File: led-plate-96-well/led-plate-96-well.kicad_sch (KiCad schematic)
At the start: 2 parts, among them U1 TLC5947RHB, U2 A000053

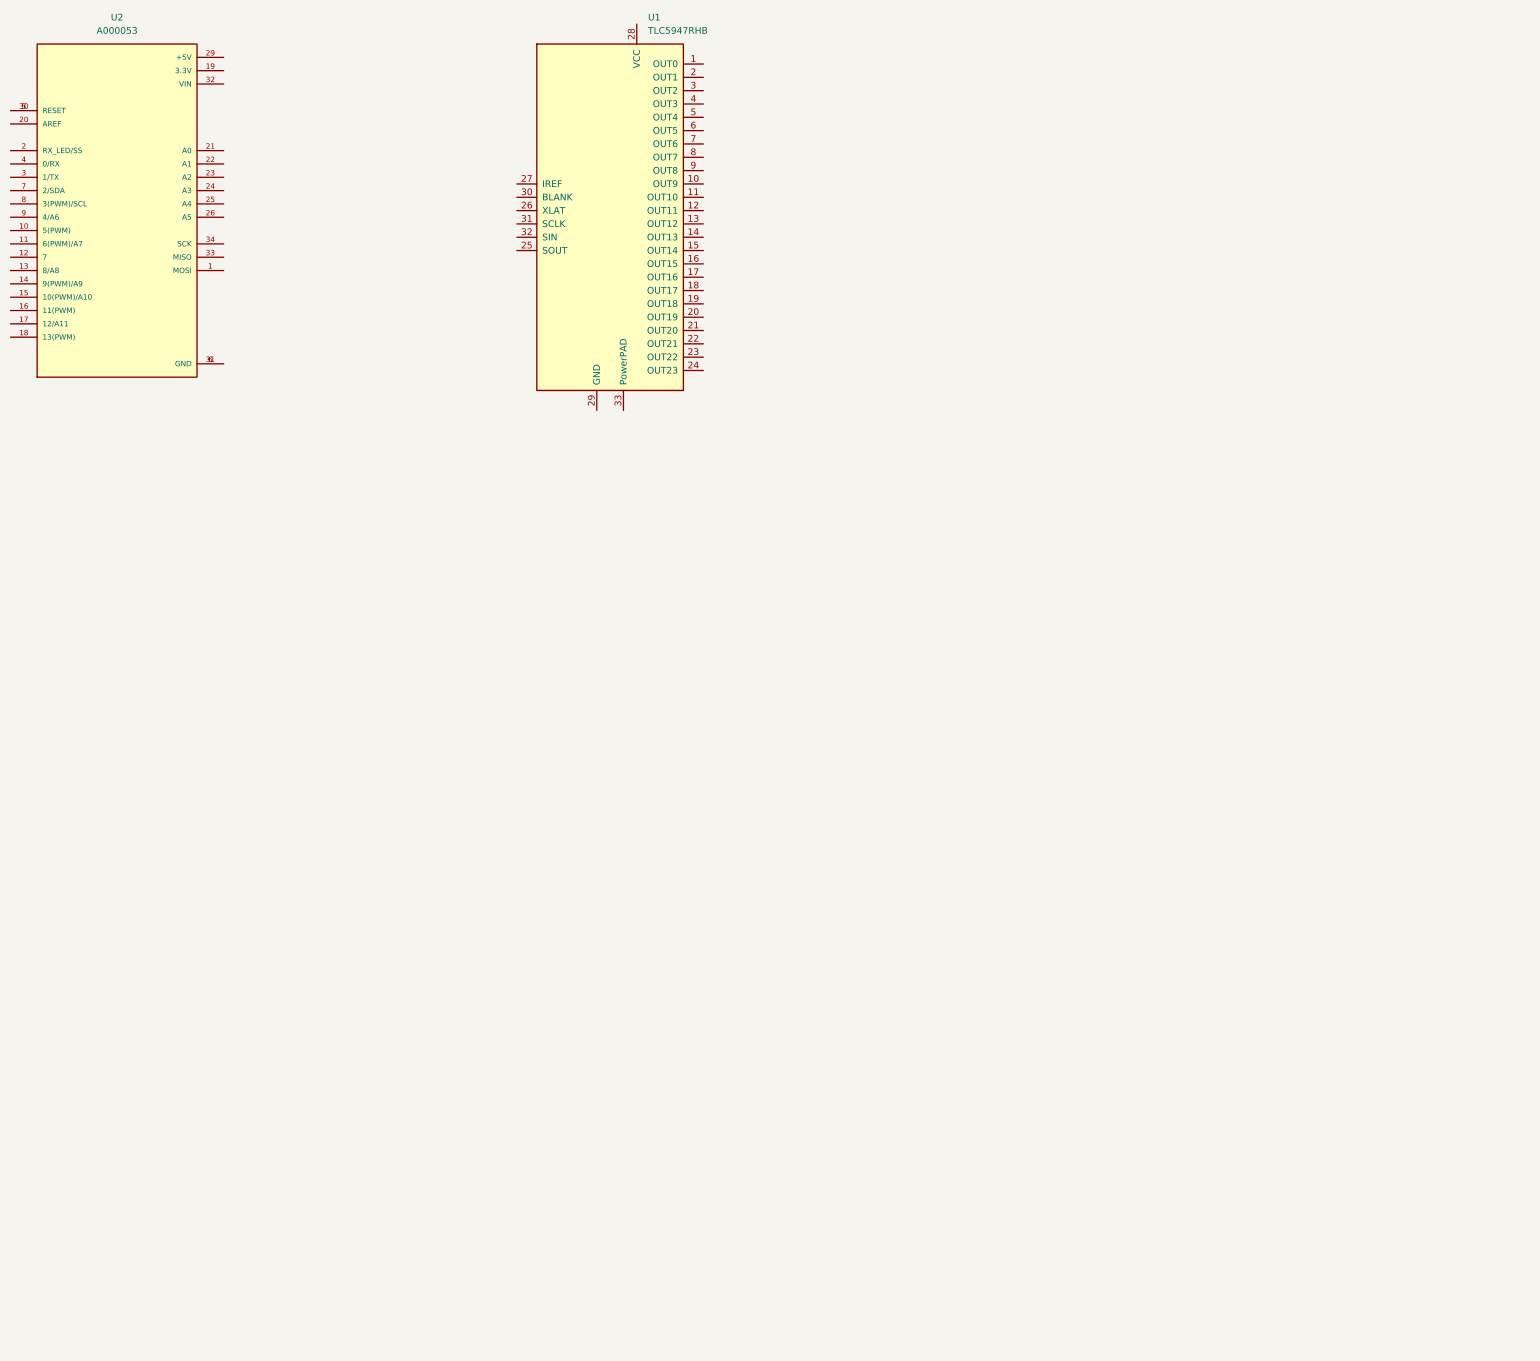
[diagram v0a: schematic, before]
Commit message: start main board
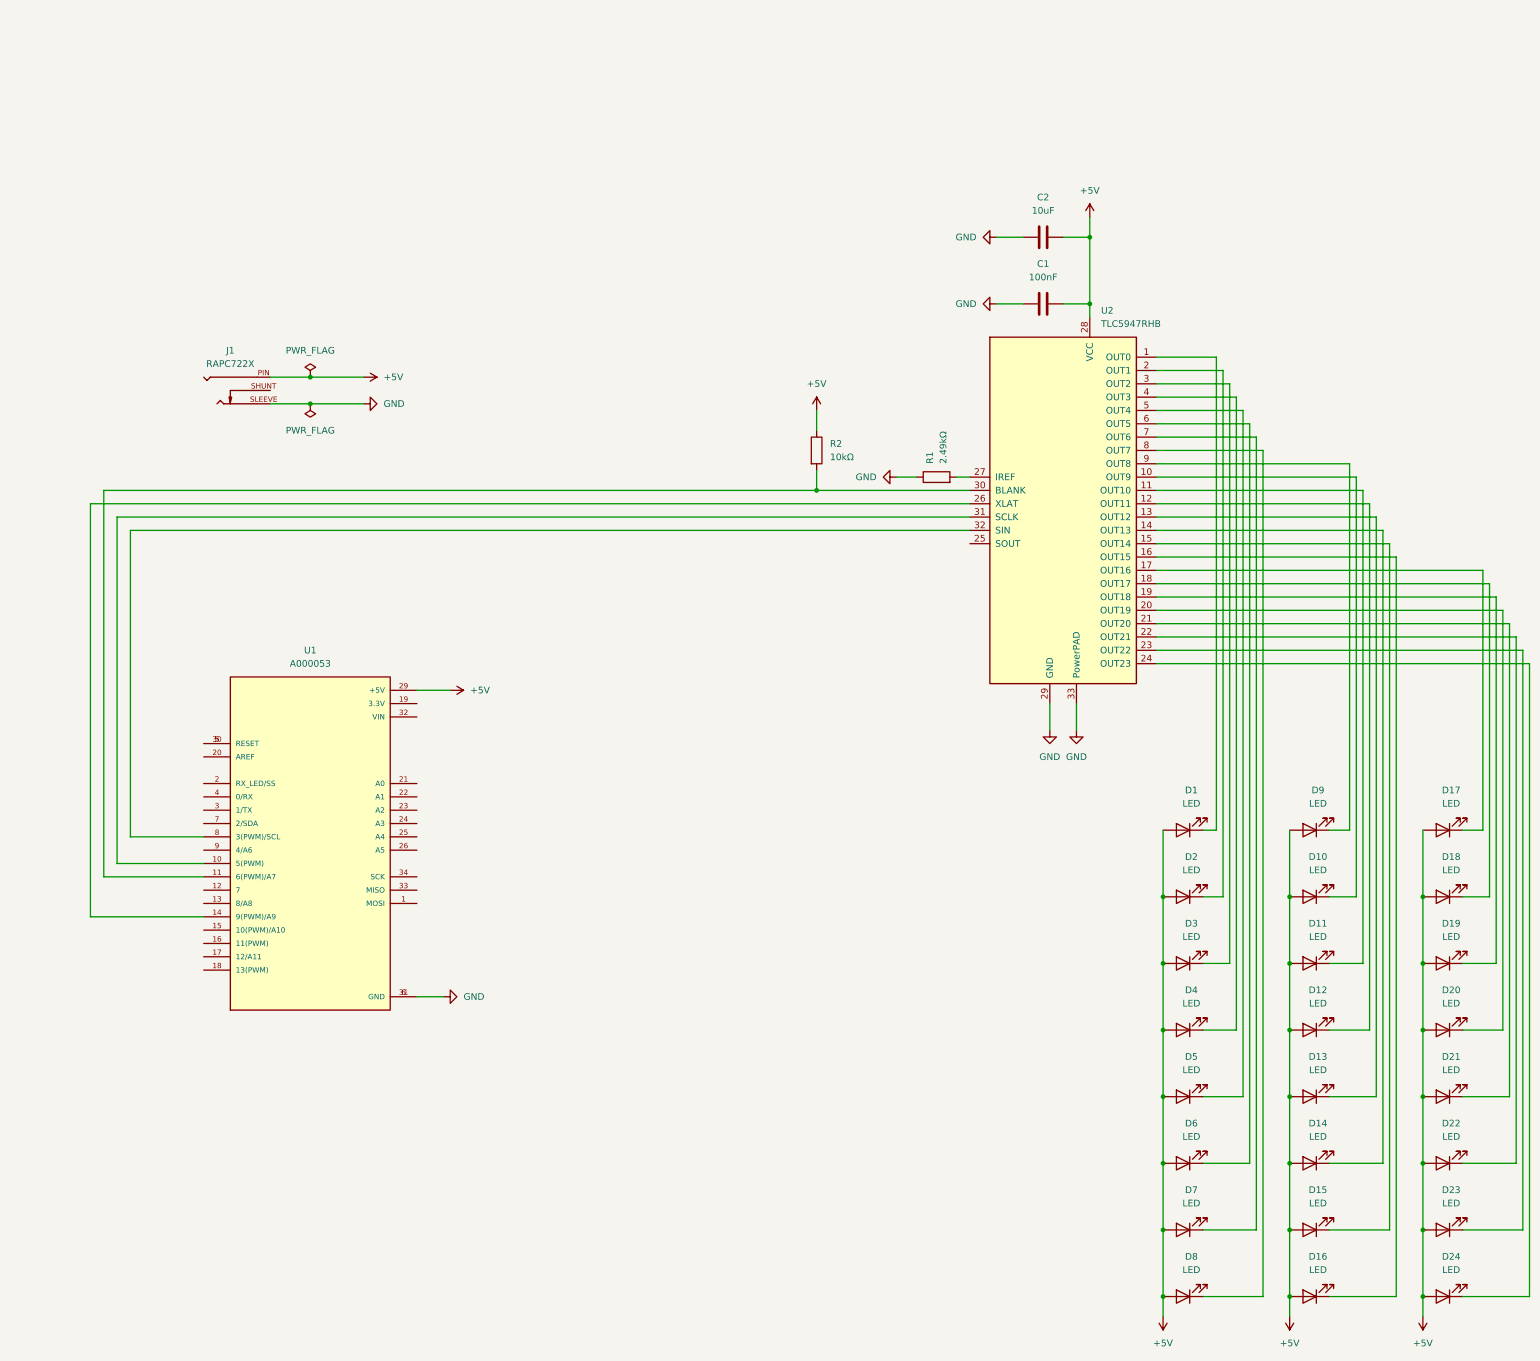
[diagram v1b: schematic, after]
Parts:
- added C1: 100nF, Capacitor_SMD:C_0603_1608Metric, symbol Device:C
- added C2: 10uF, Capacitor_SMD:C_0805_2012Metric, symbol Device:C
- added D1, D10, D11, D12, D13, D14, D15, D16, D17, D18, D19, D2, D20, D21, D22, D23, D24, D3, D4, D5, D6, D7, D8, D9: LED, SMD2835_WITH_STEP:LED_PLCC_2835, symbol Device:LED
- added J1: RAPC722X, RAPC722X:SWITCHCRAFT_RAPC722X, symbol RAPC722X:RAPC722X
- added R1: 2.49kΩ, Resistor_SMD:R_0402_1005Metric, symbol Device:R
- added R2: 10kΩ, Resistor_SMD:R_0603_1608Metric, symbol Device:R
- renumbered U2 to U1, U1 to U2
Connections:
- net at U1.10 (5(PWM)): now also U2.31 (SCLK)
- net at U1.11 (6(PWM)/A7): now also U2.30 (BLANK), R2.2
- net at U1.14 (9(PWM)/A9): now also U2.26 (XLAT)
- net +5V: now reaches U1.29 (+5V)
- net +5V: now also U2.28 (VCC), C1.2, C2.2, D1.2 (A), D10.2 (A), D11.2 (A), D12.2 (A), D13.2 (A), D14.2 (A), D15.2 (A), D16.2 (A), D17.2 (A), D18.2 (A), D19.2 (A), D2.2 (A), D20.2 (A), D21.2 (A), D22.2 (A), D23.2 (A), D24.2 (A), D3.2 (A), D4.2 (A), D5.2 (A), D6.2 (A), D7.2 (A), D8.2 (A), D9.2 (A), J1.PIN, R2.1
- net GND: now reaches U1.31 (GND), U1.6 (GND)
- net GND: now also U2.29 (GND), U2.33 (PowerPAD), C1.1, C2.1, J1.SLEEVE, R1.1
- net at U1.8 (3(PWM)/SCL): now also U2.32 (SIN)
- net at U2.1 (OUT0): now also D1.1 (K)
- net at U2.10 (OUT9): now also D10.1 (K)
- net at U2.11 (OUT10): now also D11.1 (K)
- net at U2.12 (OUT11): now also D12.1 (K)
- net at U2.13 (OUT12): now also D13.1 (K)
- net at U2.14 (OUT13): now also D14.1 (K)
- net at U2.15 (OUT14): now also D15.1 (K)
- net at U2.16 (OUT15): now also D16.1 (K)
- net at U2.17 (OUT16): now also D17.1 (K)
- net at U2.18 (OUT17): now also D18.1 (K)
- net at U2.19 (OUT18): now also D19.1 (K)
- net at U2.2 (OUT1): now also D2.1 (K)
- net at U2.20 (OUT19): now also D20.1 (K)
- net at U2.21 (OUT20): now also D21.1 (K)
- net at U2.22 (OUT21): now also D22.1 (K)
- net at U2.23 (OUT22): now also D23.1 (K)
- net at U2.24 (OUT23): now also D24.1 (K)
- net at U2.27 (IREF): now also R1.2
- net at U2.3 (OUT2): now also D3.1 (K)
- net at U2.4 (OUT3): now also D4.1 (K)
- net at U2.5 (OUT4): now also D5.1 (K)
- net at U2.6 (OUT5): now also D6.1 (K)
- net at U2.7 (OUT6): now also D7.1 (K)
- net at U2.8 (OUT7): now also D8.1 (K)
- net at U2.9 (OUT8): now also D9.1 (K)
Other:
- moved on the sheet: U1, U2
